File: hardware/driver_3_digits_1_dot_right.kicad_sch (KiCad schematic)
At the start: 11 parts, among them U4 HV5622PG

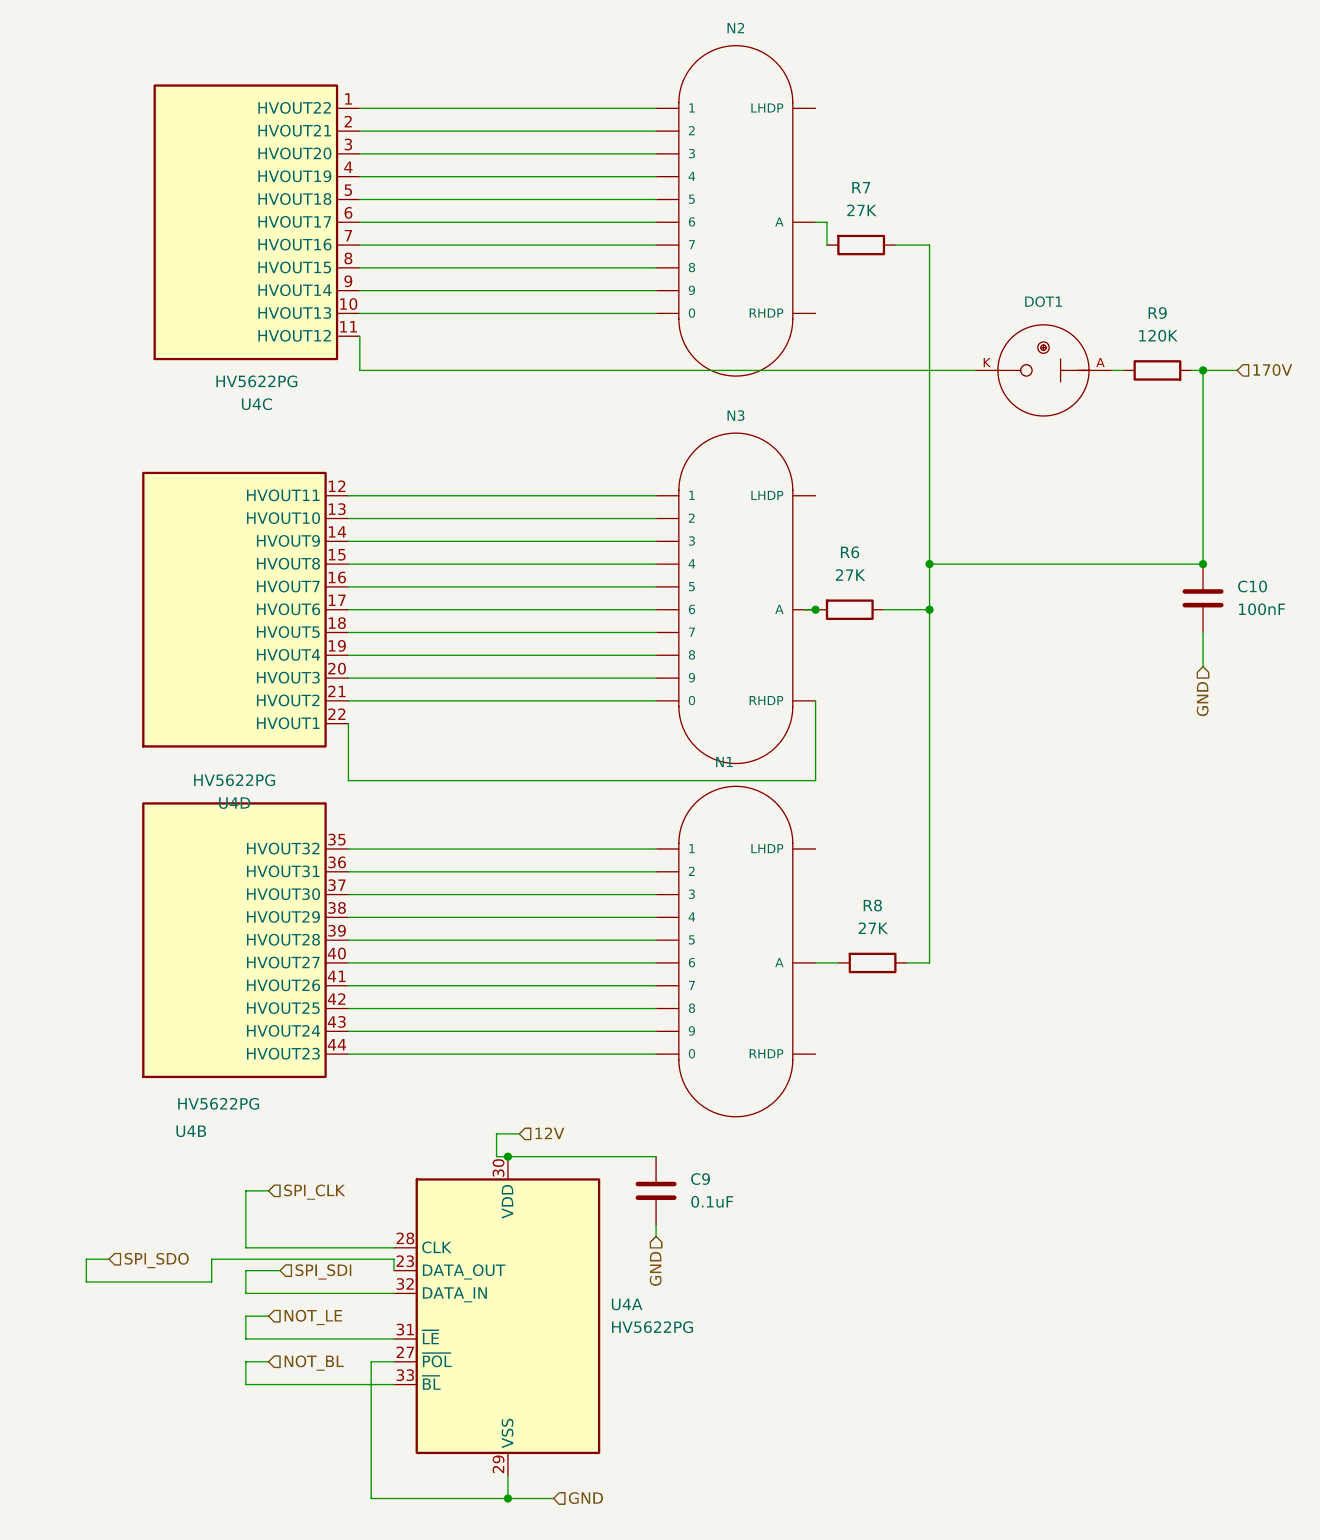
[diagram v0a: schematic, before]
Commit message: Update.
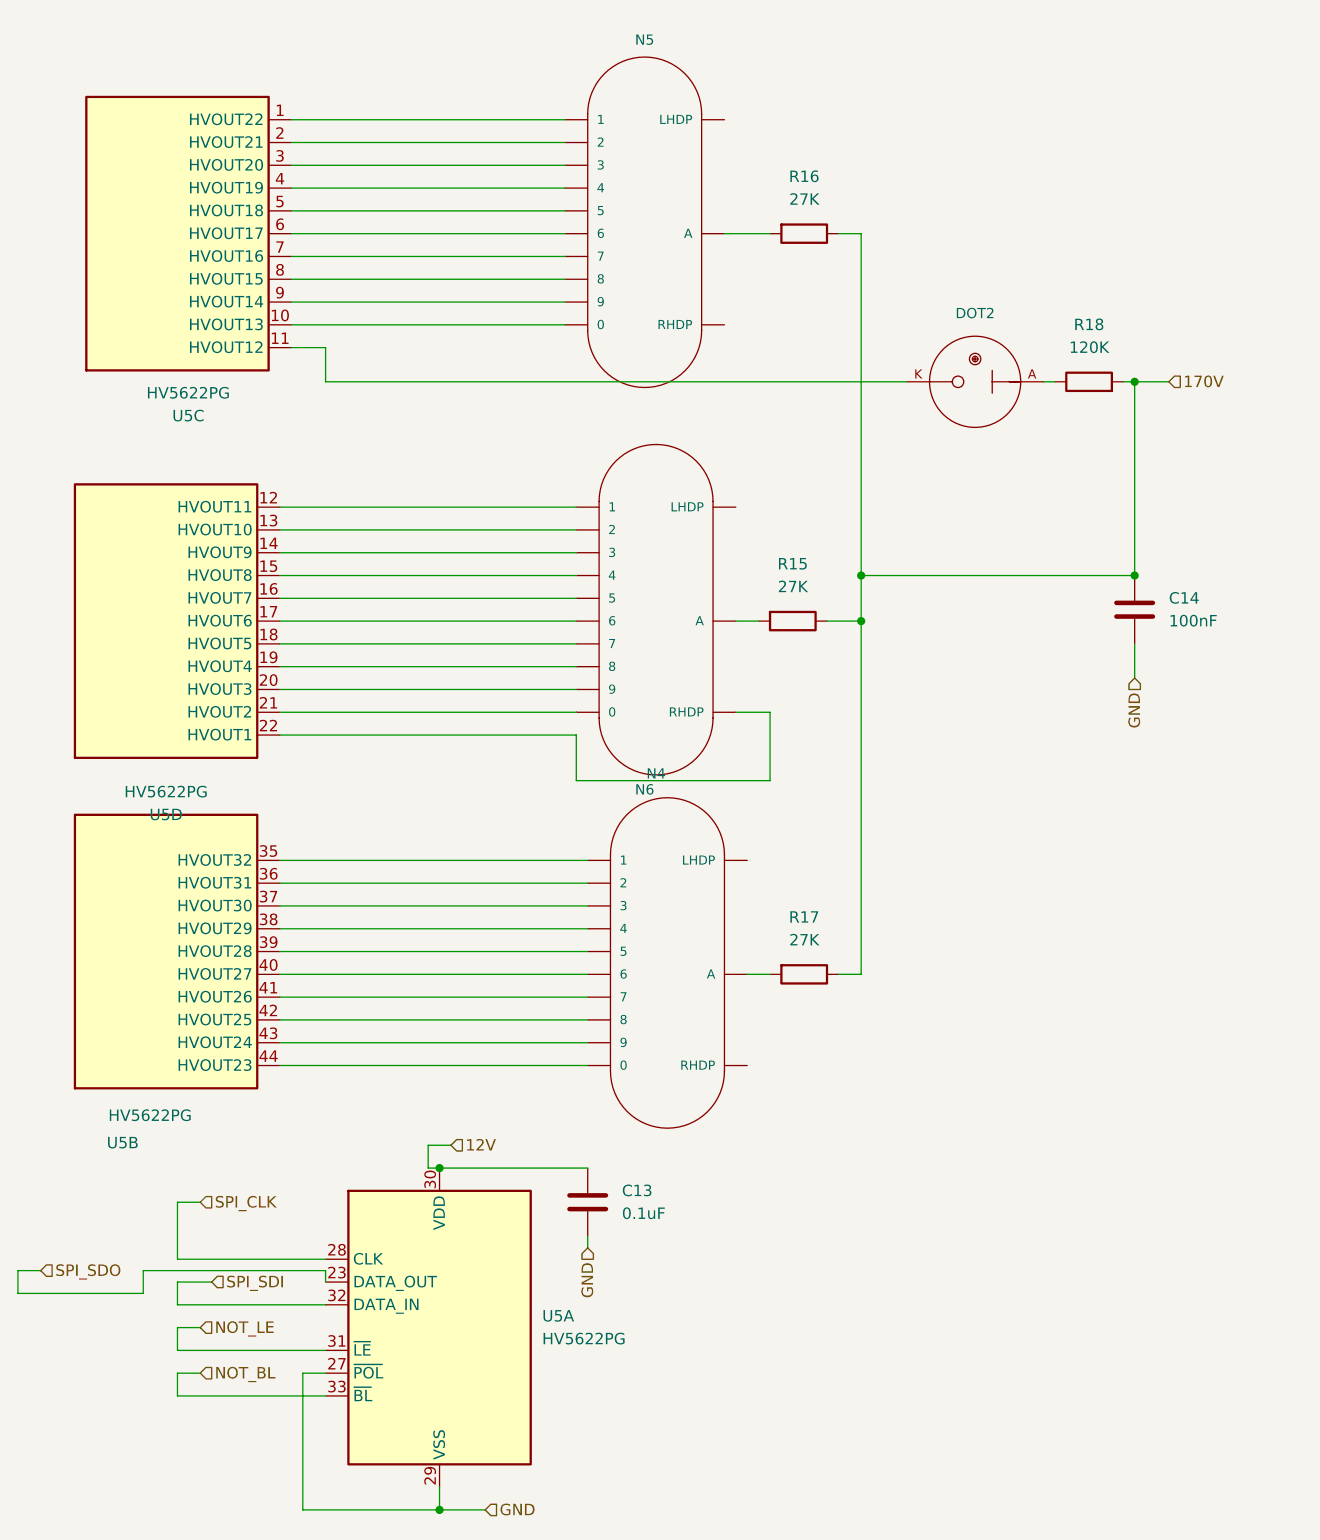
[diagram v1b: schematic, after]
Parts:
- removed C10: 100nF, Capacitor_SMD:C_1206_3216Metric, symbol Device:C
- removed C9: 0.1uF, Capacitor_SMD:C_1206_3216Metric, symbol Device:C
- removed DOT1: IN-3, nixies-us:nixies-us-IN-3, symbol nixies-us:IN-3
- removed N1, N2, N3: IN-14, nixies-us:nixies-us-IN-14, symbol nixies-us:IN-14
- removed R6, R7, R8: 27K, Resistor_SMD:R_1206_3216Metric, symbol Device:R
- removed R9: 120K, Resistor_SMD:R_1206_3216Metric, symbol Device:R
- removed U4: HV5622PG, Package_QFP:PQFP-44_10x10mm_P0.8mm, symbol HV5622:HV5622PG
- added C13: 0.1uF, Capacitor_SMD:C_1206_3216Metric, symbol Device:C
- added C14: 100nF, Capacitor_SMD:C_1206_3216Metric, symbol Device:C
- added DOT2: IN-3, nixies-us:nixies-us-IN-3, symbol nixies-us:IN-3
- added N4, N5, N6: IN-14, nixies-us:nixies-us-IN-14, symbol nixies-us:IN-14
- added R15, R16, R17: 27K, Resistor_SMD:R_1206_3216Metric, symbol Device:R
- added R18: 120K, Resistor_SMD:R_1206_3216Metric, symbol Device:R
- added U5: HV5622PG, Package_QFP:PQFP-44_10x10mm_P0.8mm, symbol HV5622:HV5622PG
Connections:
- net 12V: now also C13.2, U5.30 (VDD)
- net 170V: now also C14.1, R15.1, R16.1, R17.1, R18.2
- net GND: now also C13.1, C14.2, U5.27 (~{POL}), U5.29 (VSS)
- net NOT_BL: now also U5.33 (~{BL})
- net NOT_LE: now also U5.31 (~{LE})
- net SPI_CLK: now also U5.28 (CLK)
- net SPI_SDI: now also U5.32 (DATA_IN)
- net SPI_SDO: now also U5.23 (DATA_OUT)
- new net: N4.A, R17.2
- new net: DOT2.A, R18.1
- new net: DOT2.K, U5.11 (HVOUT12)
- new net: N5.A, R16.2
- new net: N6.A, R15.2
- new net: N5.0, U5.10 (HVOUT13)
- new net: N5.1, U5.1 (HVOUT22)
- new net: N5.2, U5.2 (HVOUT21)
- new net: N5.3, U5.3 (HVOUT20)
- new net: N5.4, U5.4 (HVOUT19)
- new net: N5.5, U5.5 (HVOUT18)
- new net: N5.6, U5.6 (HVOUT17)
- new net: N5.7, U5.7 (HVOUT16)
- new net: N5.8, U5.8 (HVOUT15)
- new net: N5.9, U5.9 (HVOUT14)
- new net: N6.0, U5.21 (HVOUT2)
- new net: N6.1, U5.12 (HVOUT11)
- new net: N6.2, U5.13 (HVOUT10)
- new net: N6.3, U5.14 (HVOUT9)
- new net: N6.4, U5.15 (HVOUT8)
- new net: N6.5, U5.16 (HVOUT7)
- new net: N6.6, U5.17 (HVOUT6)
- new net: N6.7, U5.18 (HVOUT5)
- new net: N6.8, U5.19 (HVOUT4)
- new net: N6.9, U5.20 (HVOUT3)
- new net: N6.RHDP, U5.22 (HVOUT1)
- new net: N4.0, U5.44 (HVOUT23)
- new net: N4.1, U5.35 (HVOUT32)
- new net: N4.2, U5.36 (HVOUT31)
- new net: N4.3, U5.37 (HVOUT30)
- new net: N4.4, U5.38 (HVOUT29)
- new net: N4.5, U5.39 (HVOUT28)
- new net: N4.6, U5.40 (HVOUT27)
- new net: N4.7, U5.41 (HVOUT26)
- new net: N4.8, U5.42 (HVOUT25)
- new net: N4.9, U5.43 (HVOUT24)
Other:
- title: Nixie driver for three IN-14 and one IN-3 tube -> (none)
